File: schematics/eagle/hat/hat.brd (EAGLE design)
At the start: 33 x 76.2 mm, 2 parts, among them U1 RASPBERRY_PI_3B+_HDRMODEL_RAS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

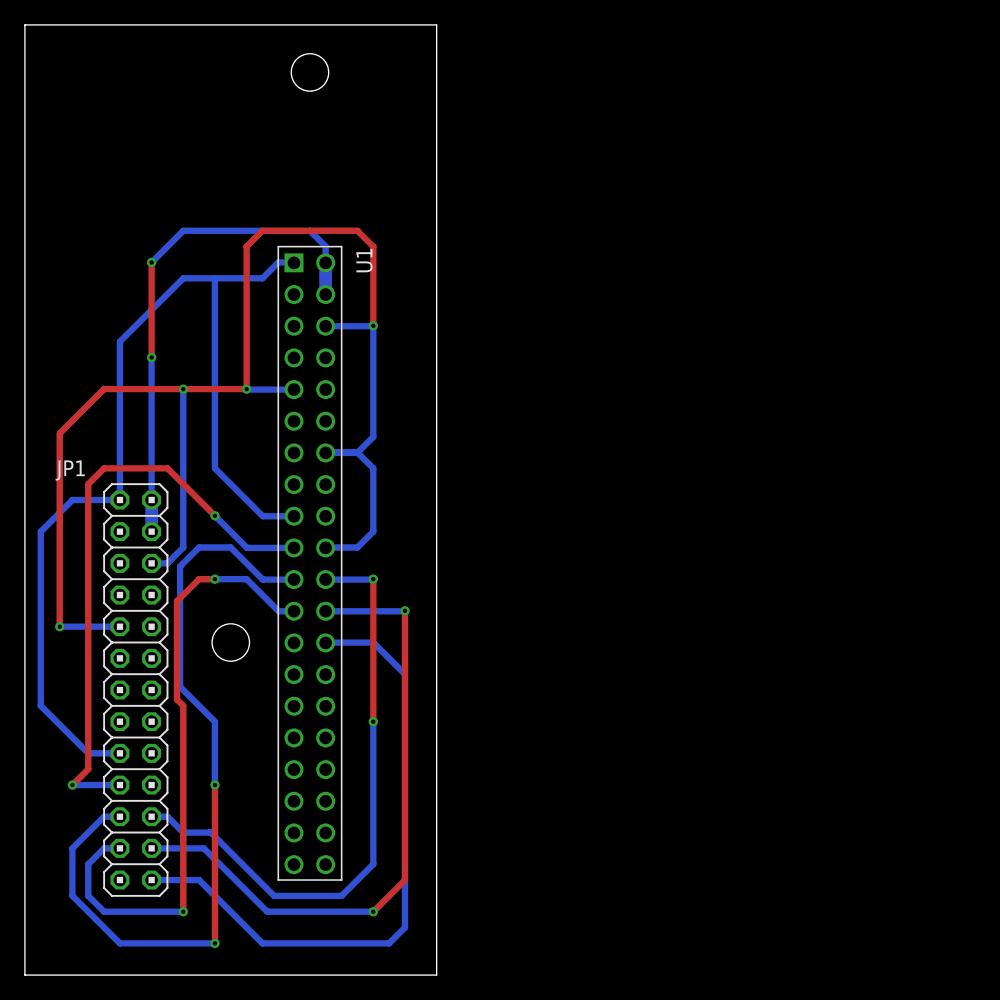
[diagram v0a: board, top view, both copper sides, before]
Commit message: reorg
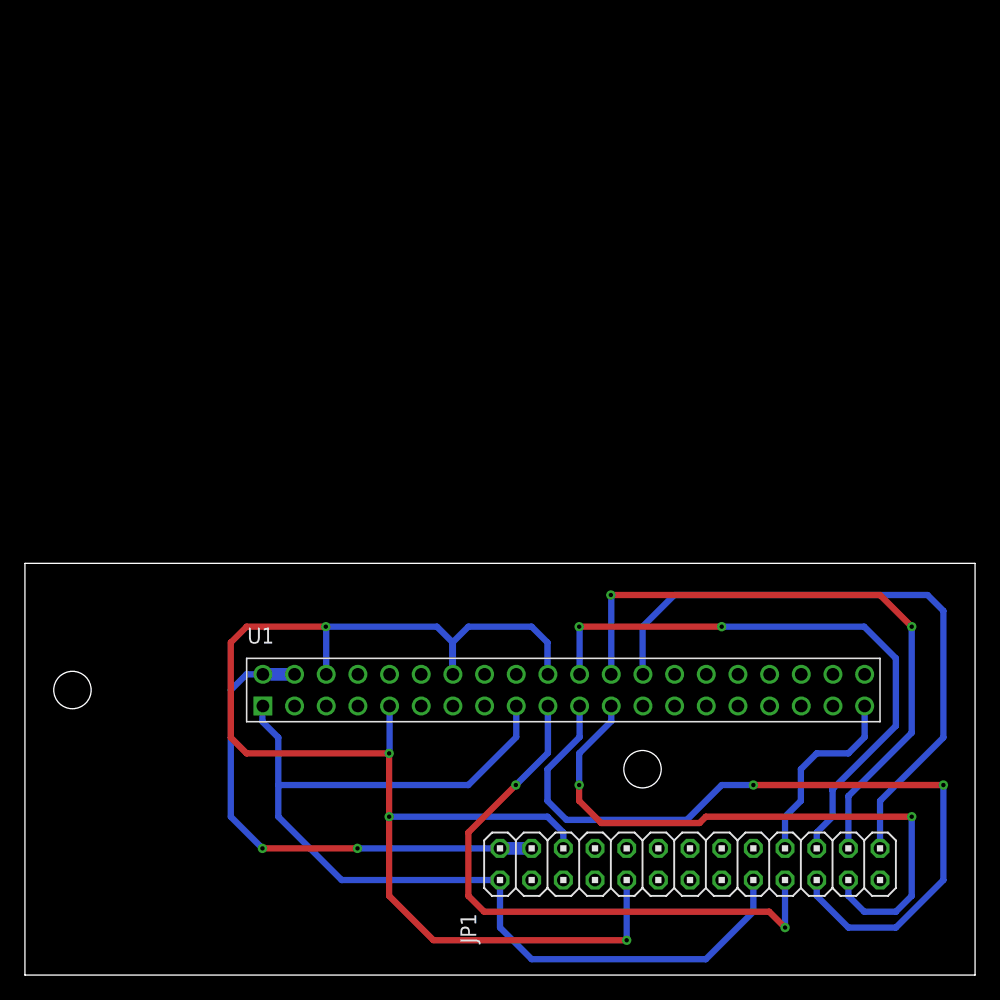
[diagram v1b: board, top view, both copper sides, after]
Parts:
- moved JP1 46.6 mm to (53.3, 8.89), turned to 0 degrees
- moved U1 35.7 mm to (19.1, 21.6), turned to 0 degrees
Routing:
- net GND: track 116.2 -> 131.8 mm
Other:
- board size 33 x 76.2 mm -> 76.2 x 33 mm
